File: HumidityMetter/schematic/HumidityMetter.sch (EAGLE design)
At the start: 2 parts

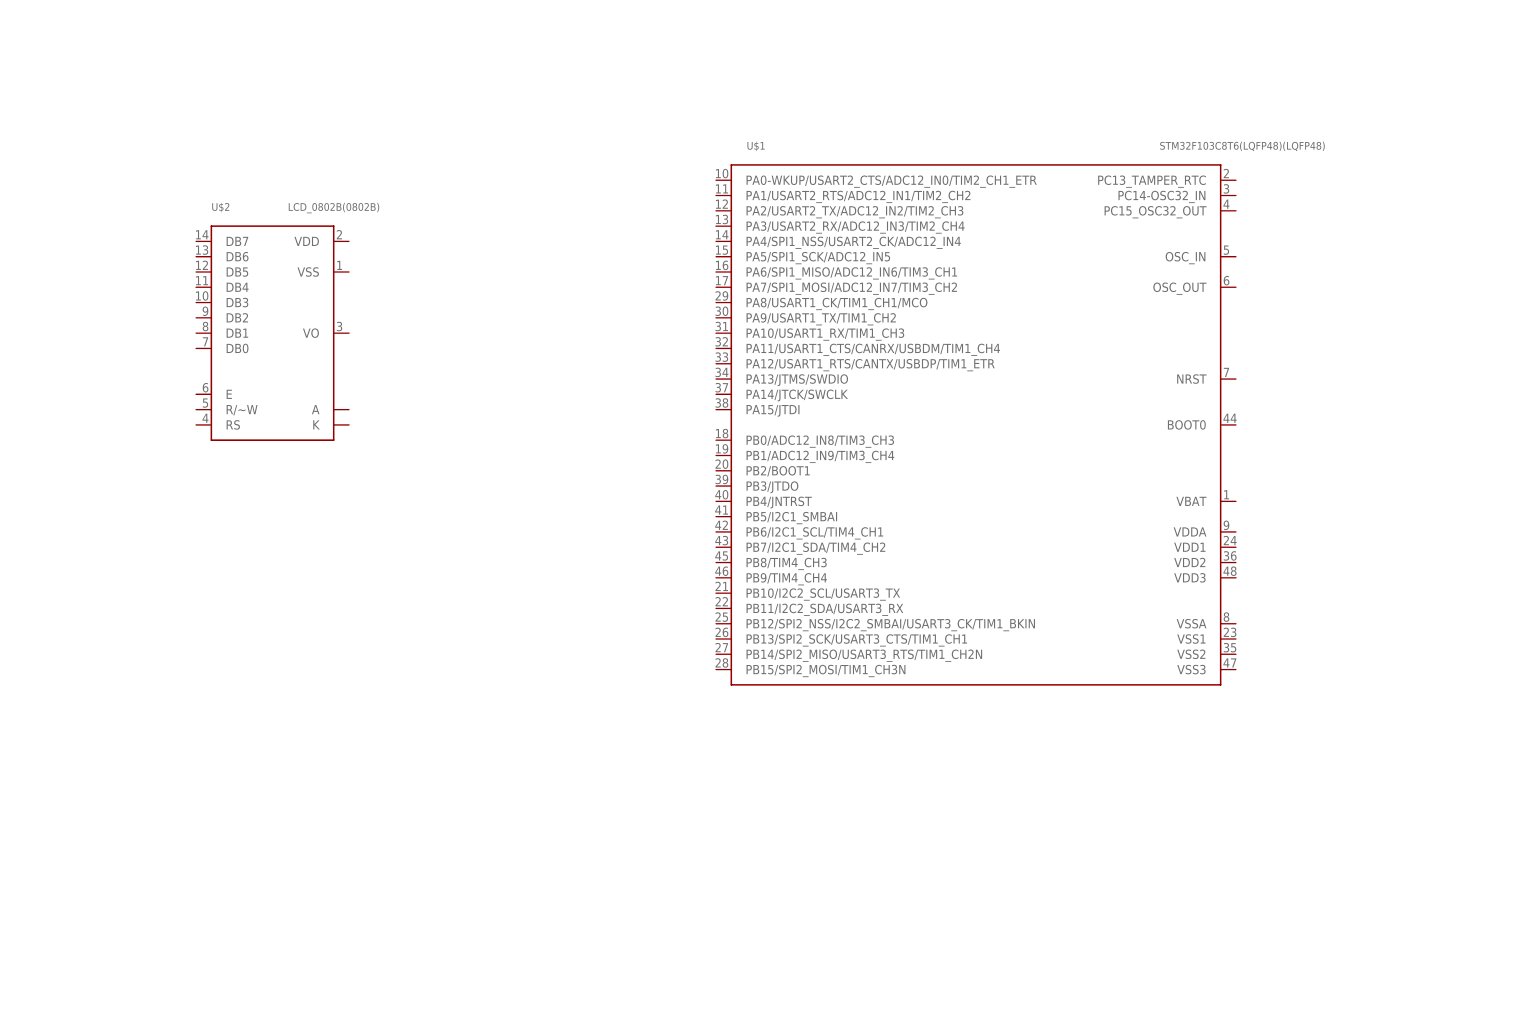
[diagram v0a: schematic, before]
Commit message: Humidity metter. Start schematic routing.
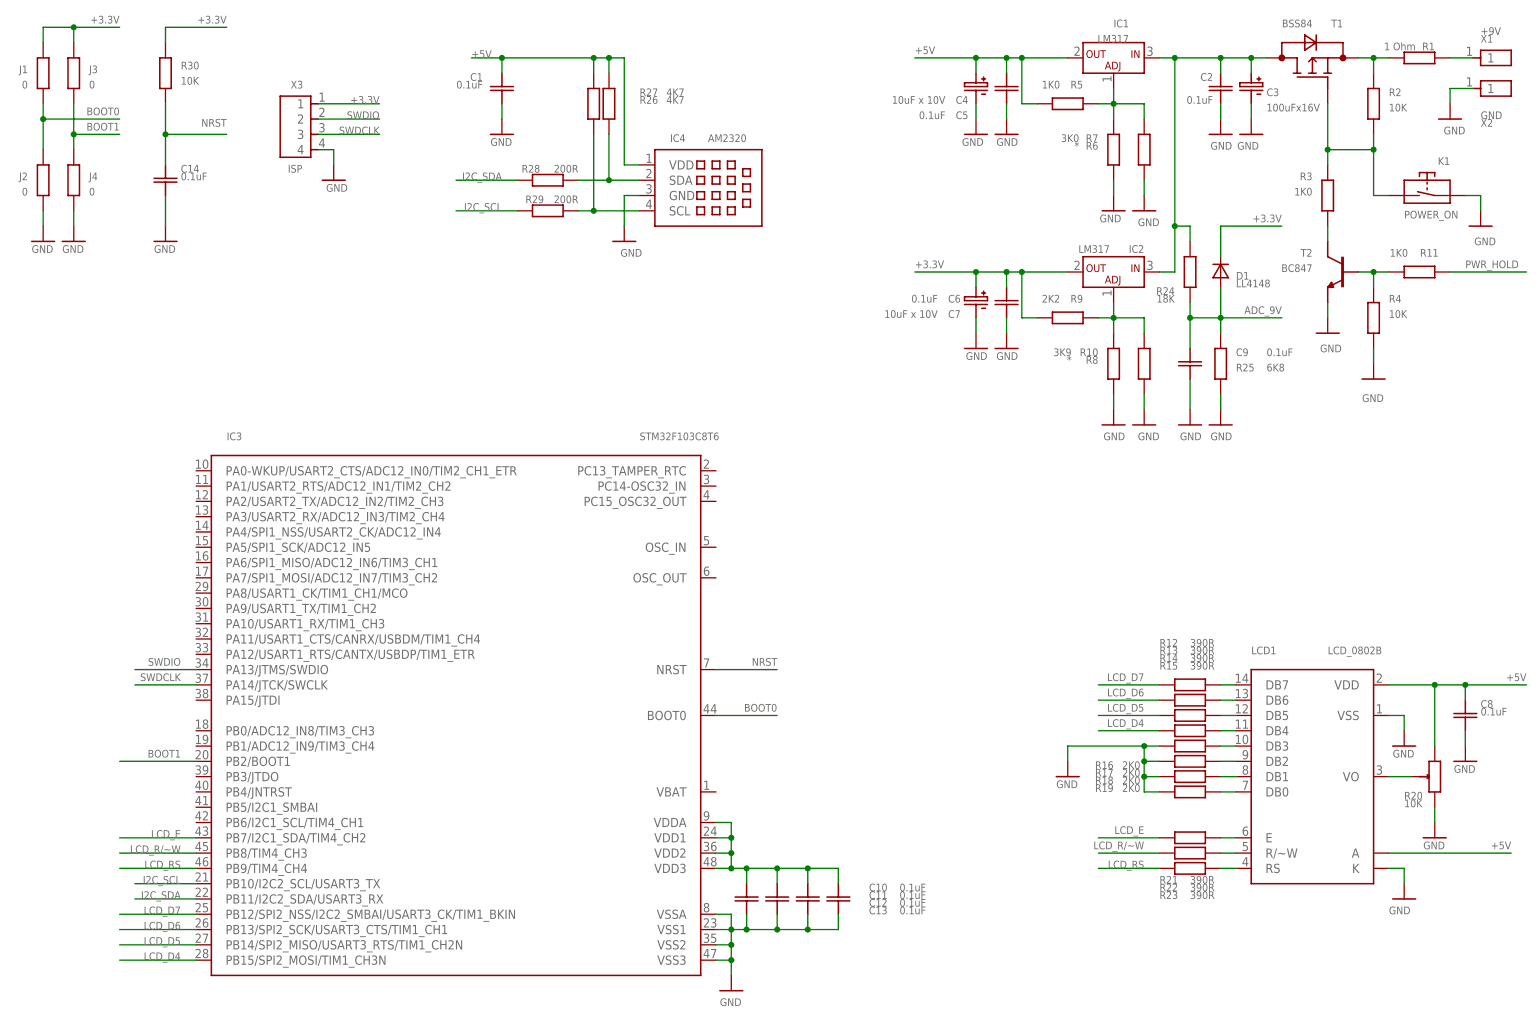
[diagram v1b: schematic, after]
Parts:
- removed U$1: STM32F103C8T6(LQFP48)(LQFP48), __MyCommonLib1:STM32F103C8T6(LQFP48)(LQFP48)
- removed U$2: LCD_0802B(0802B), __MyCommonLib1:LCD_0802B(0802B)
- added C1, C10, C11, C12, C13, C14, C2, C5, C6, C8, C9: 0.1uF, __MyCommonLib1:CSMD_0805
- added C3: 100uFx16V, __MyCommonLib1:CE6.3MM
- added C4, C7: 10uF x 10V, __MyCommonLib1:CE5.2MM
- added D1: LL4148, __MyCommonLib1:LL4147SOD-80
- added IC1, IC2: LM317, __MyCommonLib1:LM317(D2PAK)
- added IC3: STM32F103C8T6, __MyCommonLib1:STM32F103C8T6(LQFP48)(LQFP48)
- added IC4: AM2320, __MyCommonLib1:AM2320(HOR)
- added J1, J2, J3, J4: 0, __MyCommonLib1:RSMD_0805
- added K1: POWER_ON, __MyCommonLib1:KEY(7X4.5)
- added LCD1: LCD_0802B, __MyCommonLib1:LCD_0802B(0802B)
- added R1: 1 Ohm, __MyCommonLib1:RSMD_1206
- added R10: 3K9, __MyCommonLib1:RSMD_0805
- added R11, R3, R5: 1K0, __MyCommonLib1:RSMD_0805
- added R12, R13, R14, R15, R21, R22, R23: 390R, __MyCommonLib1:RSMD_0805
- added R16, R17, R18, R19: 2K0, __MyCommonLib1:RSMD_0805
- added R2, R30, R4: 10K, __MyCommonLib1:RSMD_0805
- added R20: 10K, __MyCommonLib1:R_ADJSTAND_6.5_X_3.5MM
- added R24: 18K, __MyCommonLib1:RSMD_0805
- added R25: 6K8, __MyCommonLib1:RSMD_0805
- added R26, R27: 4K7, __MyCommonLib1:RSMD_0805
- added R28, R29: 200R, __MyCommonLib1:RSMD_0805
- added R6, R8: *, __MyCommonLib1:RSMD_0805
- added R7: 3K0, __MyCommonLib1:RSMD_0805
- added R9: 2K2, __MyCommonLib1:RSMD_0805
- added T1: BSS84, __MyCommonLib1:BSS84(SOT23)
- added T2: BC847, __MyCommonLib1:BC847SOT23_SMALL_PADS
- added X1: +9V, __MyCommonLib1:PIN1X13.5MM_DRILL
- added X2: GND, __MyCommonLib1:PIN1X13.5MM_DRILL
- added X3: ISP, __MyCommonLib1:PIN4X1(2.54MM)
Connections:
- new net +3.3V: C6.PIN1, C7.PLUS, D1.CATHODE, IC2.OUT, J1.PIN0, J3.PIN0, R30.PIN0, R9.PIN1, X3.1
- new net +5V: C1.PIN1, C4.PLUS, C5.PIN1, C8.PIN1, IC1.OUT, IC4.VDD, LCD1.A, LCD1.VDD, R20.END_A, R26.PIN0, R27.PIN0, R5.PIN1
- new net ADC_9V: C9.PIN1, D1.ANODE, R24.PIN1, R25.PIN0
- new net BOOT0: IC3.BOOT0, J1.PIN1, J2.PIN0
- new net BOOT1: IC3.PB2/BOOT1, J3.PIN1, J4.PIN0
- new net GND: C1.PIN0, C10.PIN0, C11.PIN0, C12.PIN0, C13.PIN0, C14.PIN0, C2.PIN0, C3.MINUS, C4.MINUS, C5.PIN0, C6.PIN0, C7.MINUS, C8.PIN0, C9.PIN0, IC3.VSS1, IC3.VSS2, IC3.VSS3, IC3.VSSA, IC4.GND, J2.PIN1, J4.PIN1, K1.1, LCD1.K, LCD1.VSS, R10.PIN1, R16.PIN1, R17.PIN1, R18.PIN1, R19.PIN1, R20.END_B, R25.PIN1, R4.PIN1, R6.PIN1, R7.PIN1, R8.PIN1, T2.E, X2.1, X3.4
- new net I2C_SCL: IC3.PB10/I2C2_SCL/USART3_TX, R29.PIN0
- new net I2C_SDA: IC3.PB11/I2C2_SDA/USART3_RX, R28.PIN0
- new net LCD_D4: IC3.PB15/SPI2_MOSI/TIM1_CH3N, R15.PIN1
- new net LCD_D5: IC3.PB14/SPI2_MISO/USART3_RTS/TIM1_CH2N, R14.PIN1
- new net LCD_D6: IC3.PB13/SPI2_SCK/USART3_CTS/TIM1_CH1, R13.PIN1
- new net LCD_D7: IC3.PB12/SPI2_NSS/I2C2_SMBAI/USART3_CK/TIM1_BKIN, R12.PIN1
- new net LCD_E: IC3.PB7/I2C1_SDA/TIM4_CH2, R21.PIN1
- new net LCD_R/~W: IC3.PB8/TIM4_CH3, R22.PIN1
- new net LCD_RS: IC3.PB9/TIM4_CH4, R23.PIN1
- new net N$1: R1.PIN1, X1.1
- new net N$10: LCD1.DB7, R12.PIN0
- new net N$11: LCD1.DB6, R13.PIN0
- new net N$12: LCD1.DB5, R14.PIN0
- new net N$13: LCD1.DB4, R15.PIN0
- new net N$14: IC4.SDA, R26.PIN1, R28.PIN1
- new net N$15: LCD1.DB3, R16.PIN0
- new net N$16: LCD1.DB2, R17.PIN0
- new net N$17: LCD1.DB1, R18.PIN0
- new net N$18: LCD1.DB0, R19.PIN0
- new net N$19: C10.PIN1, C11.PIN1, C12.PIN1, C13.PIN1, IC3.VDD1, IC3.VDD2, IC3.VDD3, IC3.VDDA
- new net N$2: R1.PIN0, R2.PIN0, T1.SOURCE
- new net N$20: IC4.SCL, R27.PIN1, R29.PIN1
- new net N$21: LCD1.RS, R23.PIN0
- new net N$22: LCD1.R/~W, R22.PIN0
- new net N$23: LCD1.E, R21.PIN0
- new net N$3: K1.2, R2.PIN1, R3.PIN0, T1.GATE
- new net N$4: R3.PIN1, T2.C
- new net N$5: R11.PIN1, R4.PIN0, T2.B
- new net N$6: C2.PIN1, C3.PLUS, IC1.IN, IC2.IN, R24.PIN0, T1.DRAIN
- new net N$7: IC1.ADJ, R5.PIN0, R6.PIN0, R7.PIN0
- new net N$8: IC2.ADJ, R10.PIN0, R8.PIN0, R9.PIN0
- new net N$9: LCD1.VO, R20.ADJ
- new net NRST: C14.PIN1, IC3.NRST, R30.PIN1
- new net PWR_HOLD: R11.PIN0
- new net SWDCLK: IC3.PA14/JTCK/SWCLK, X3.3
- new net SWDIO: IC3.PA13/JTMS/SWDIO, X3.2
